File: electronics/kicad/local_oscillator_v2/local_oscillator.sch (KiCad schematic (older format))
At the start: 23 parts, among them P2 TestPoint:TestPoint_Pad_1.5x1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, P3 TestPoint:TestPoint_Pad_1.5x1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, U1 CE3520K3

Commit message: Notch filter
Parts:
- removed C3, C?: 10 pF, 0402, symbol SparkFun-Capacitors:6PF-0402-50V-0.5%
- removed D1, D? (x3): D, Diode_SMD:D_SOD-523, symbol Device:D
- removed D?: D_Capacitance, Diode_SMD:D_SOD-523, symbol Device:D_Capacitance
- removed P? (x6): TestPoint:TestPoint_Pad_1.5x1.5mm, TestPoint:TestPoint_Pad_3.0x3.0mm, symbol conn:CONN_1
- removed TP1: SMA, TestPoint:TestPoint_Pad_1.5x1.5mm, symbol SparkFun-Connectors:TEST-POINT3X4
- removed U?: CE3520K3, 0xDBFB7:4-Micro-X, symbol 0xDBFB7:CE3520K3
- added C1: 1 pF, 0402, symbol SparkFun-Capacitors:6PF-0402-50V-0.5%
- added P1, P5, P6, P7: TestPoint:TestPoint_Pad_1.5x1.5mm, TestPoint:TestPoint_Pad_3.0x3.0mm, symbol conn:CONN_1
- added P4: TestPoint:TestPoint_Pad_1.5x1.5mm, TestPoint:TestPoint_Pad_1.5x1.5mm, symbol conn:CONN_1
- added R1, R2, R3: 50 Ohm, 0603, symbol SparkFun-Resistors:RESISTOR0603
- C2: renamed from C?; value 10 pF -> 1 pF
- P2, P3: footprint TestPoint:TestPoint_Pad_1.5x1.5mm -> TestPoint:TestPoint_Pad_3.0x3.0mm
- gave numbers to parts that had none: 1
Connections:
- net labels removed: GATE
- wire segments 27 -> 17
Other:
- moved on the sheet: C2, C6, D1

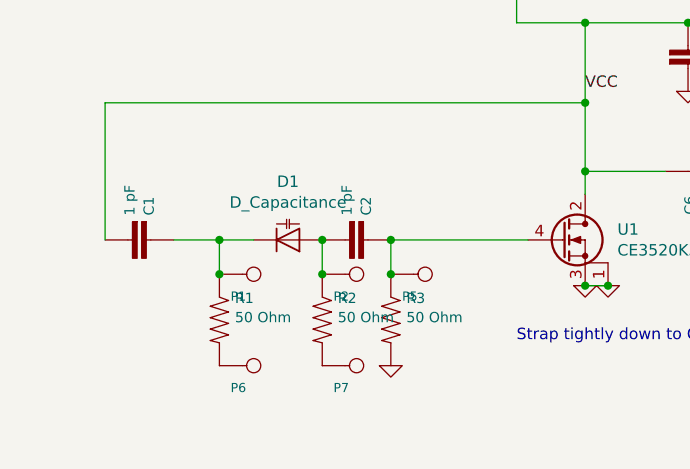
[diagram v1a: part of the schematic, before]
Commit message: aaaaaaaaaaaa
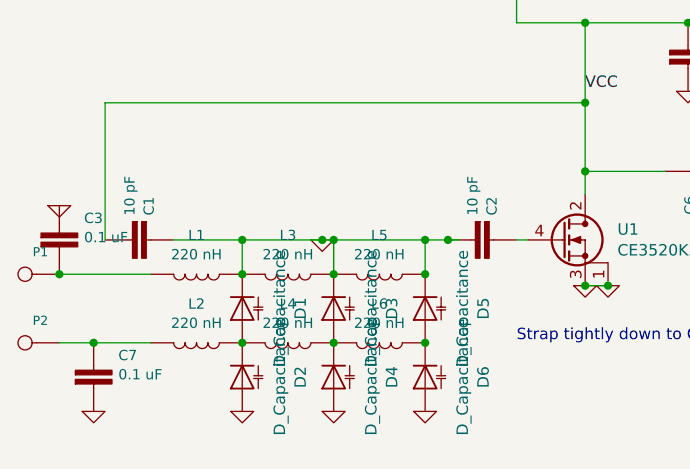
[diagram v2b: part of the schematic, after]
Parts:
- removed P5, P6, P7: TestPoint:TestPoint_Pad_1.5x1.5mm, TestPoint:TestPoint_Pad_3.0x3.0mm, symbol conn:CONN_1
- removed R1, R2, R3: 50 Ohm, 0603, symbol SparkFun-Resistors:RESISTOR0603
- added C3, C7: 0.1 uF, 0603, symbol SparkFun-Capacitors:4.7UF0603
- added D2, D3, D4, D5, D6: D_Capacitance, Diode_SMD:D_SOD-523, symbol Device:D_Capacitance
- added L1, L2, L3, L4, L5, L6: 220 nH, 0402, symbol SparkFun-Coils:INDUCTOR-0402-3.9NH
- C1, C2: value 1 pF -> 10 pF
- P1, P2, P3: footprint TestPoint:TestPoint_Pad_3.0x3.0mm -> TestPoint:TestPoint_Pad_1.5x1.5mm
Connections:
- wire segments 17 -> 24

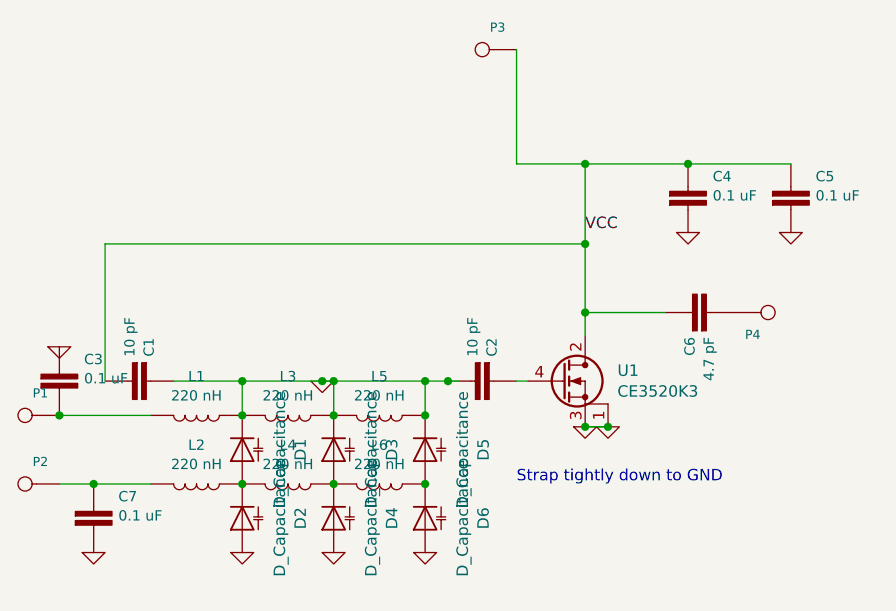
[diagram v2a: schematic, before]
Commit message: goddamnit
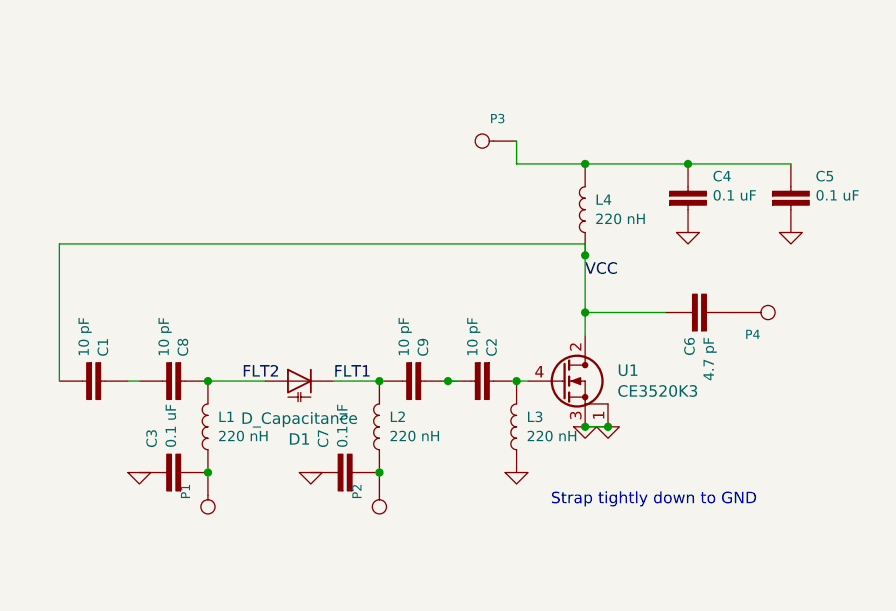
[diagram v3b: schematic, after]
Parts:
- removed D2, D3, D4, D5, D6: D_Capacitance, Diode_SMD:D_SOD-523, symbol Device:D_Capacitance
- removed L5, L6: 220 nH, 0402, symbol SparkFun-Coils:INDUCTOR-0402-3.9NH
- added C8, C9: 10 pF, 0402, symbol SparkFun-Capacitors:6PF-0402-50V-0.5%
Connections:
- net labels added: FLT1, FLT2
- wire segments 24 -> 16
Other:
- moved on the sheet: C1, P3

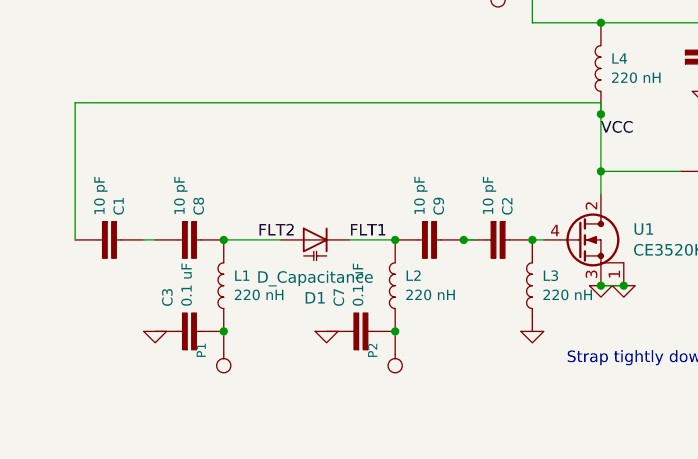
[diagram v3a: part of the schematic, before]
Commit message: Colpitts? huh
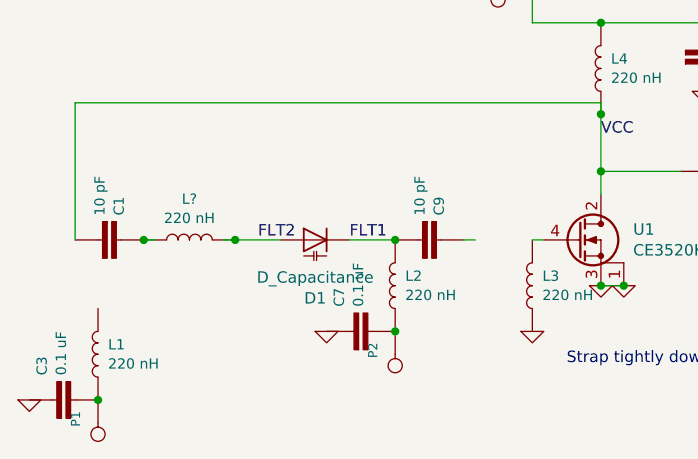
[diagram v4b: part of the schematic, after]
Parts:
- removed C2, C8: 10 pF, 0402, symbol SparkFun-Capacitors:6PF-0402-50V-0.5%
- added L?: 220 nH, 0402, symbol SparkFun-Coils:INDUCTOR-0402-3.9NH
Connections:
- wire segments 16 -> 17
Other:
- moved on the sheet: C3, L1, P1
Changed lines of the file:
@@
 	5400 4650 5350 4650
-$Comp
-L SparkFun-Capacitors:6PF-0402-50V-0.5% C2
-U 1 1 5EBF9629
-P 5250 4650
-F 0 "C2" H 5143 4658 45  0000 R CNN
-F 1 "10 pF" H 5143 4742 45  0000 R CNN
-F 2 "0402" H 5250 4900 20  0001 C CNN
-F 3 "" H 5250 4650 50  0001 C CNN
-F 4 "" H 5143 4784 60  0000 R CNN "Field4"
-	1    5250 4650
-	0    -1   1    0
-$EndComp
 $Comp
 L conn:CONN_1 P3
@@
 Wire Wire Line
 	5050 4650 5100 4650
-Connection ~ 5350 4650
 $Comp
 L power:GND #PWR0105
@@
 L SparkFun-Coils:INDUCTOR-0402-3.9NH L1
 U 1 1 5EC4BEE4
-P 4000 4850
-F 0 "L1" H 3956 4808 45  0000 R CNN
-F 1 "220 nH" H 3956 4892 45  0000 R CNN
-F 2 "0402" H 4000 5100 20  0001 C CNN
-F 3 "" H 4000 4850 50  0001 C CNN
-F 4 "" H 4052 4766 60  0000 L CNN "Field4"
-	1    4000 4850
-	-1   0    0    1
-$EndComp
-Wire Wire Line
-	4000 4650 4250 4650
+P 3450 5150
+F 0 "L1" H 3406 5108 45  0000 R CNN
+F 1 "220 nH" H 3406 5192 45  0000 R CNN
+F 2 "0402" H 3450 5400 20  0001 C CNN
+F 3 "" H 3450 5150 50  0001 C CNN
+F 4 "" H 3502 5066 60  0000 L CNN "Field4"
+	1    3450 5150
+	-1   0    0    1
+$EndComp
+Wire Wire Line
+	4000 4650 4050 4650
 Text Label 4550 4650 0    50   ~ 0
 FLT1
@@
 L conn:CONN_1 P1
 U 1 1 5EC655E9
-P 4000 5200
-F 0 "P1" H 3933 5103 40  0000 C CNN
-F 1 "TestPoint:TestPoint_Pad_1.5x1.5mm" H 3950 5240 30  0001 C CNN
-F 2 "TestPoint:TestPoint_Pad_1.5x1.5mm" H 4000 5200 50  0001 C CNN
-F 3 "" H 4000 5200 50  0001 C CNN
-	1    4000 5200
+P 3450 5500
+F 0 "P1" H 3383 5403 40  0000 C CNN
+F 1 "TestPoint:TestPoint_Pad_1.5x1.5mm" H 3400 5540 30  0001 C CNN
+F 2 "TestPoint:TestPoint_Pad_1.5x1.5mm" H 3450 5500 50  0001 C CNN
+F 3 "" H 3450 5500 50  0001 C CNN
+	1    3450 5500
 	0    1    1    0
 $EndComp
@@
 L SparkFun-Capacitors:4.7UF0603 C3
 U 1 1 5EC67FE6
-P 3900 5050
-F 0 "C3" H 4008 5195 45  0000 L CNN
-F 1 "0.1 uF" H 4008 5111 45  0000 L CNN
-F 2 "0603" H 3900 5300 20  0001 C CNN
-F 3 "" H 3900 5050 50  0001 C CNN
-F 4 "CAP-08280" V 4008 5016 60  0001 L CNN "Field4"
-	1    3900 5050
+P 3350 5350
+F 0 "C3" H 3458 5495 45  0000 L CNN
+F 1 "0.1 uF" H 3458 5411 45  0000 L CNN
+F 2 "0603" H 3350 5600 20  0001 C CNN
+F 3 "" H 3350 5350 50  0001 C CNN
+F 4 "CAP-08280" V 3458 5316 60  0001 L CNN "Field4"
+	1    3350 5350
 	0    -1   -1   0
 $EndComp
-Connection ~ 4000 5050
+Connection ~ 3450 5350
 $Comp
 L power:GND #PWR0106
 U 1 1 5EC69CEA
-P 3700 5050
-F 0 "#PWR0106" H 3700 5050 30  0001 C CNN
-F 1 "GND" H 3700 4980 30  0001 C CNN
-F 2 "" H 3700 5050 50  0001 C CNN
-F 3 "" H 3700 5050 50  0001 C CNN
-	1    3700 5050
+P 3150 5350
+F 0 "#PWR0106" H 3150 5350 30  0001 C CNN
+F 1 "GND" H 3150 5280 30  0001 C CNN
+F 2 "" H 3150 5350 50  0001 C CNN
+F 3 "" H 3150 5350 50  0001 C CNN
+	1    3150 5350
 	1    0    0    -1
 $EndComp
@@
 $EndComp
 Connection ~ 4750 4650
-Connection ~ 5050 4650
 Wire Wire Line
 	3350 4050 5650 4050
-$Comp
-L SparkFun-Capacitors:6PF-0402-50V-0.5% C8
-U 1 1 5EC77179
-P 3900 4650
-F 0 "C8" H 3793 4658 45  0000 R CNN
-F 1 "10 pF" H 3793 4742 45  0000 R CNN
-F 2 "0402" H 3900 4900 20  0001 C CNN
-F 3 "" H 3900 4650 50  0001 C CNN
-F 4 "" H 3793 4784 60  0000 R CNN "Field4"
-	1    3900 4650
-	0    -1   1    0
-$EndComp
-Connection ~ 4000 4650
 Wire Wire Line
 	3650 4650 3700 4650
+$Comp
+L SparkFun-Coils:INDUCTOR-0402-3.9NH L?
+U 1 1 5EC8409C
+P 3850 4650
+F 0 "L?" V 4029 4650 45  0000 C CNN
+F 1 "220 nH" V 3945 4650 45  0000 C CNN
+F 2 "0402" H 3850 4900 20  0001 C CNN
+F 3 "" H 3850 4650 50  0001 C CNN
+F 4 "" H 3902 4566 60  0000 L CNN "Field4"
+	1    3850 4650
+	0    -1   -1   0
+$EndComp
+Connection ~ 3650 4650
+Connection ~ 4050 4650
+Wire Wire Line
+	4050 4650 4250 4650
 $EndSCHEMATC

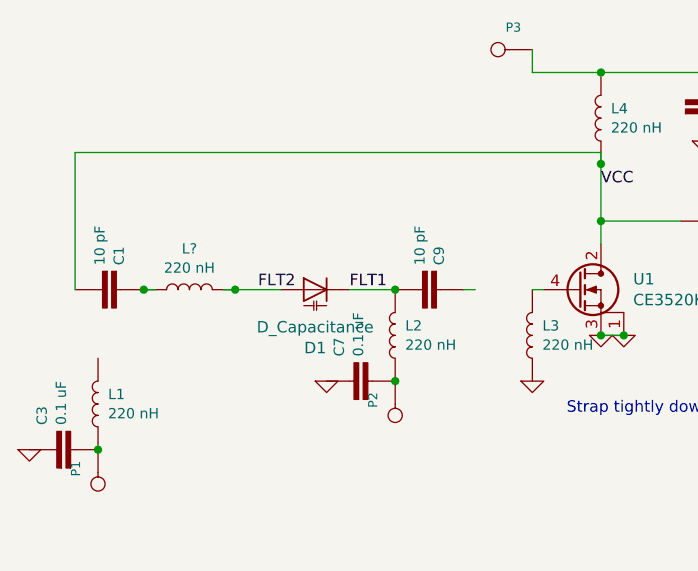
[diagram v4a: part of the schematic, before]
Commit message: Inductance
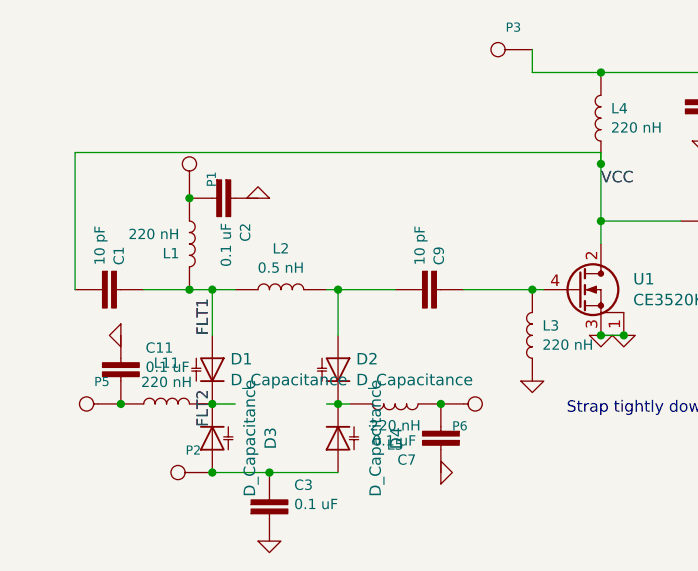
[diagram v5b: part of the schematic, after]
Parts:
- removed L2: 220 nH, 0402, symbol SparkFun-Coils:INDUCTOR-0402-3.9NH
- added C11, C2: 0.1 uF, 0603, symbol SparkFun-Capacitors:4.7UF0603
- added D2, D3, D4: D_Capacitance, Diode_SMD:D_SOD-523, symbol Device:D_Capacitance
- added L11, L5: 220 nH, 0402, symbol SparkFun-Coils:INDUCTOR-0402-3.9NH
- added P5, P6: TestPoint:TestPoint_Pad_1.5x1.5mm, TestPoint:TestPoint_Pad_1.5x1.5mm, symbol conn:CONN_1
- L2: renamed from L?; value 220 nH -> 0.5 nH
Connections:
- wire segments 17 -> 25
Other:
- moved on the sheet: D1, L2

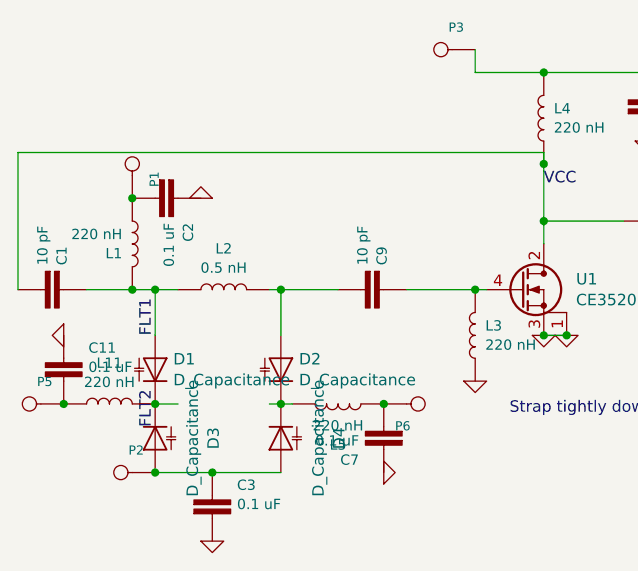
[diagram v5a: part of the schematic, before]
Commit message: <chef's kiss>
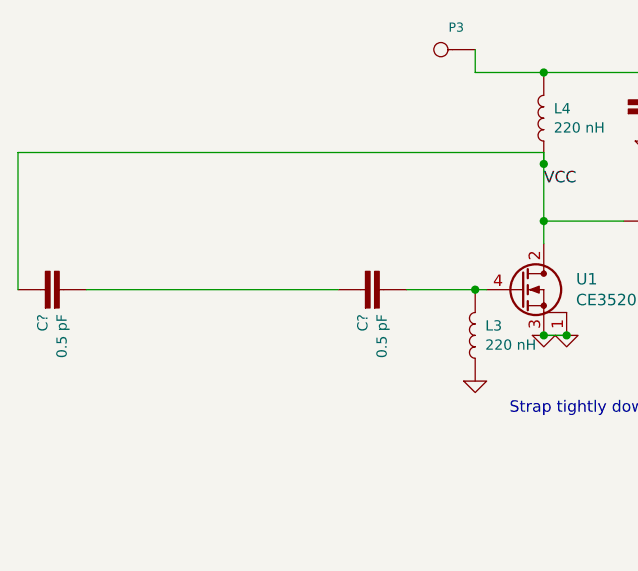
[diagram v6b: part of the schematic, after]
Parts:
- removed C1, C9: 10 pF, 0402, symbol SparkFun-Capacitors:6PF-0402-50V-0.5%
- removed C11, C2, C3, C7: 0.1 uF, 0603, symbol SparkFun-Capacitors:4.7UF0603
- removed D1, D2, D3, D4: D_Capacitance, Diode_SMD:D_SOD-523, symbol Device:D_Capacitance
- removed L1, L11, L5: 220 nH, 0402, symbol SparkFun-Coils:INDUCTOR-0402-3.9NH
- removed L2: 0.5 nH, 0402, symbol SparkFun-Coils:INDUCTOR-0402-3.9NH
- removed P1, P2, P5, P6: TestPoint:TestPoint_Pad_1.5x1.5mm, TestPoint:TestPoint_Pad_1.5x1.5mm, symbol conn:CONN_1
- added C? (x2): 0.5 pF, 0402, symbol SparkFun-Capacitors:6PF-0402-50V-0.5%
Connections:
- net labels removed: FLT1, FLT2
- wire segments 25 -> 14

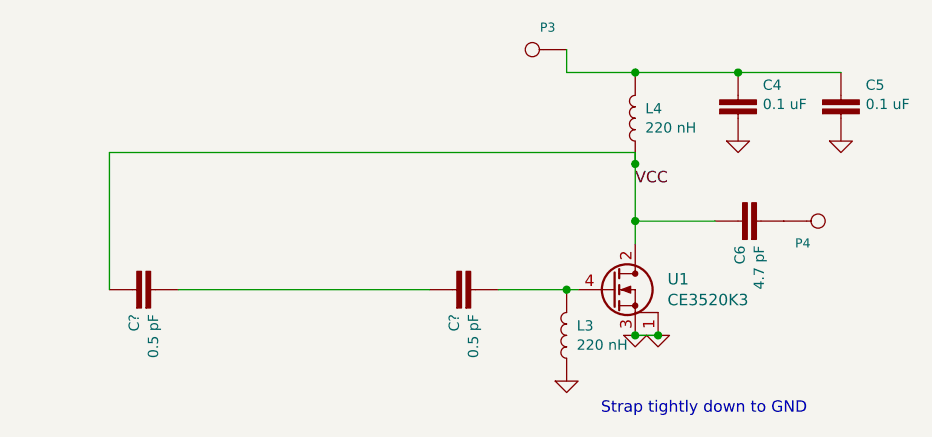
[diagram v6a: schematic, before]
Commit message: Rewrking board
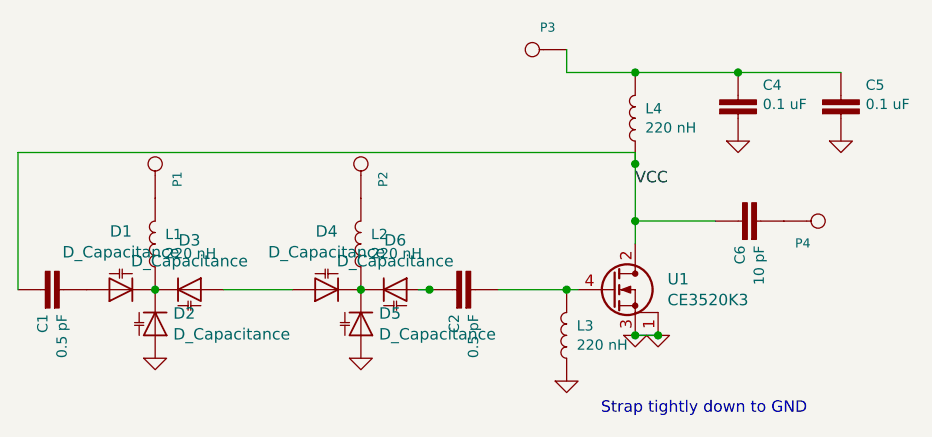
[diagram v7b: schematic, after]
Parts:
- added D1, D2, D3, D4, D5, D6: D_Capacitance, Diode_SMD:D_SOD-523, symbol Device:D_Capacitance
- added L1, L2: 220 nH, 0402, symbol SparkFun-Coils:INDUCTOR-0402-3.9NH
- added P1, P2: TestPoint:TestPoint_Pad_1.5x1.5mm, TestPoint:TestPoint_Pad_1.5x1.5mm, symbol conn:CONN_1
- C6: value 4.7 pF -> 10 pF
- gave numbers to parts that had none: 2
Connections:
- wire segments 14 -> 15
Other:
- moved on the sheet: C1
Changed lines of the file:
@@
 P 6100 4350
 F 0 "C6" H 5993 4358 45  0000 R CNN
-F 1 "4.7 pF" H 5993 4442 45  0000 R CNN
+F 1 "10 pF" H 5993 4442 45  0000 R CNN
 F 2 "0402" H 6100 4600 20  0001 C CNN
 F 3 "" H 6100 4350 50  0001 C CNN
@@
 Wire Wire Line
 	5350 3600 5350 3700
-Wire Wire Line
-	3350 4050 5650 4050
-$Comp
-L SparkFun-Capacitors:6PF-0402-50V-0.5% C?
+$Comp
+L SparkFun-Capacitors:6PF-0402-50V-0.5% C1
 U 1 1 5ED0CDE7
-P 3450 4650
-F 0 "C?" H 3343 4658 45  0000 R CNN
-F 1 "0.5 pF" H 3343 4742 45  0000 R CNN
-F 2 "0402" H 3450 4900 20  0001 C CNN
-F 3 "" H 3450 4650 50  0001 C CNN
-F 4 "" H 3343 4784 60  0000 R CNN "Field4"
-	1    3450 4650
+P 3050 4650
+F 0 "C1" H 2943 4658 45  0000 R CNN
+F 1 "0.5 pF" H 2943 4742 45  0000 R CNN
+F 2 "0402" H 3050 4900 20  0001 C CNN
+F 3 "" H 3050 4650 50  0001 C CNN
+F 4 "" H 2943 4784 60  0000 R CNN "Field4"
+	1    3050 4650
 	0    1    -1   0
 $EndComp
-$Comp
-L SparkFun-Capacitors:6PF-0402-50V-0.5% C?
+Connection ~ 5350 4650
+Wire Wire Line
+	2950 4650 2950 4050
+$Comp
+L Device:D_Capacitance D4
+U 1 1 5ED19DD8
+P 4300 4650
+F 0 "D4" H 4300 4395 50  0000 C CNN
+F 1 "D_Capacitance" H 4300 4486 50  0000 C CNN
+F 2 "Diode_SMD:D_SOD-523" H 4300 4650 50  0001 C CNN
+F 3 "~" H 4300 4650 50  0001 C CNN
+	1    4300 4650
+	-1   0    0    1
+$EndComp
+Wire Wire Line
+	5050 4650 5350 4650
+$Comp
+L Device:D_Capacitance D6
+U 1 1 5ED15CAF
+P 4600 4650
+F 0 "D6" H 4600 4866 50  0000 C CNN
+F 1 "D_Capacitance" H 4600 4775 50  0000 C CNN
+F 2 "Diode_SMD:D_SOD-523" H 4600 4650 50  0001 C CNN
+F 3 "~" H 4600 4650 50  0001 C CNN
+	1    4600 4650
+	1    0    0    -1
+$EndComp
+Wire Wire Line
+	4750 4650 4700 4650
+$Comp
+L SparkFun-Capacitors:6PF-0402-50V-0.5% C2
 U 1 1 5ED0E8E1
 P 4850 4650
-F 0 "C?" H 4743 4658 45  0000 R CNN
+F 0 "C2" H 4743 4658 45  0000 R CNN
 F 1 "0.5 pF" H 4743 4742 45  0000 R CNN
 F 2 "0402" H 4850 4900 20  0001 C CNN
@@
 	0    1    -1   0
 $EndComp
-Wire Wire Line
-	5050 4650 5350 4650
-Connection ~ 5350 4650
-Wire Wire Line
-	4750 4650 3650 4650
-Wire Wire Line
-	3350 4650 3350 4050
+Connection ~ 4750 4650
+$Comp
+L Device:D_Capacitance D3
+U 1 1 5ED12D3F
+P 3700 4650
+F 0 "D3" H 3700 4866 50  0000 C CNN
+F 1 "D_Capacitance" H 3700 4775 50  0000 C CNN
+F 2 "Diode_SMD:D_SOD-523" H 3700 4650 50  0001 C CNN
+F 3 "~" H 3700 4650 50  0001 C CNN
+	1    3700 4650
+	1    0    0    -1
+$EndComp
+$Comp
+L Device:D_Capacitance D5
+U 1 1 5ED164DA
+P 4450 4800
+F 0 "D5" V 4404 4879 50  0000 L CNN
+F 1 "D_Capacitance" V 4495 4879 50  0000 L CNN
+F 2 "Diode_SMD:D_SOD-523" H 4450 4800 50  0001 C CNN
+F 3 "~" H 4450 4800 50  0001 C CNN
+	1    4450 4800
+	0    1    1    0
+$EndComp
+$Comp
+L power:GND #PWR0106
+U 1 1 5ED177E8
+P 4450 4950
+F 0 "#PWR0106" H 4450 4950 30  0001 C CNN
+F 1 "GND" H 4450 4880 30  0001 C CNN
+F 2 "" H 4450 4950 50  0001 C CNN
+F 3 "" H 4450 4950 50  0001 C CNN
+	1    4450 4950
+	1    0    0    -1
+$EndComp
+Connection ~ 3550 4650
+$Comp
+L Device:D_Capacitance D1
+U 1 1 5ED19292
+P 3400 4650
+F 0 "D1" H 3400 4395 50  0000 C CNN
+F 1 "D_Capacitance" H 3400 4486 50  0000 C CNN
+F 2 "Diode_SMD:D_SOD-523" H 3400 4650 50  0001 C CNN
+F 3 "~" H 3400 4650 50  0001 C CNN
+	1    3400 4650
+	-1   0    0    1
+$EndComp
+$Comp
+L power:GND #PWR0107
+U 1 1 5ED14708
+P 3550 4950
+F 0 "#PWR0107" H 3550 4950 30  0001 C CNN
+F 1 "GND" H 3550 4880 30  0001 C CNN
+F 2 "" H 3550 4950 50  0001 C CNN
+F 3 "" H 3550 4950 50  0001 C CNN
+	1    3550 4950
+	1    0    0    -1
+$EndComp
+$Comp
+L Device:D_Capacitance D2
+U 1 1 5ED0FC00
+P 3550 4800
+F 0 "D2" V 3504 4879 50  0000 L CNN
+F 1 "D_Capacitance" V 3595 4879 50  0000 L CNN
+F 2 "Diode_SMD:D_SOD-523" H 3550 4800 50  0001 C CNN
+F 3 "~" H 3550 4800 50  0001 C CNN
+	1    3550 4800
+	0    1    1    0
+$EndComp
+Wire Wire Line
+	2950 4050 5650 4050
+Connection ~ 4450 4650
+Wire Wire Line
+	4150 4650 3850 4650
+$Comp
+L SparkFun-Coils:INDUCTOR-0402-3.9NH L2
+U 1 1 5ED2E2A3
+P 4450 4450
+F 0 "L2" H 4406 4408 45  0000 R CNN
+F 1 "220 nH" H 4406 4492 45  0000 R CNN
+F 2 "0402" H 4450 4700 20  0001 C CNN
+F 3 "" H 4450 4450 50  0001 C CNN
+F 4 "" H 4502 4366 60  0000 L CNN "Field4"
+	1    4450 4450
+	-1   0    0    1
+$EndComp
+$Comp
+L SparkFun-Coils:INDUCTOR-0402-3.9NH L1
+U 1 1 5ED2EEFE
+P 3550 4450
+F 0 "L1" H 3506 4408 45  0000 R CNN
+F 1 "220 nH" H 3506 4492 45  0000 R CNN
+F 2 "0402" H 3550 4700 20  0001 C CNN
+F 3 "" H 3550 4450 50  0001 C CNN
+F 4 "" H 3602 4366 60  0000 L CNN "Field4"
+	1    3550 4450
+	-1   0    0    1
+$EndComp
+$Comp
+L conn:CONN_1 P2
+U 1 1 5ED2FA6B
+P 4450 4100
+F 0 "P2" H 4383 4003 40  0000 C CNN
+F 1 "TestPoint:TestPoint_Pad_1.5x1.5mm" H 4400 4140 30  0001 C CNN
+F 2 "TestPoint:TestPoint_Pad_1.5x1.5mm" H 4450 4100 50  0001 C CNN
+F 3 "" H 4450 4100 50  0001 C CNN
+	1    4450 4100
+	0    -1   -1   0
+$EndComp
+$Comp
+L conn:CONN_1 P1
+U 1 1 5ED30ECA
+P 3550 4100
+F 0 "P1" H 3483 4003 40  0000 C CNN
+F 1 "TestPoint:TestPoint_Pad_1.5x1.5mm" H 3500 4140 30  0001 C CNN
+F 2 "TestPoint:TestPoint_Pad_1.5x1.5mm" H 3550 4100 50  0001 C CNN
+F 3 "" H 3550 4100 50  0001 C CNN
+	1    3550 4100
+	0    -1   -1   0
+$EndComp
 $EndSCHEMATC
